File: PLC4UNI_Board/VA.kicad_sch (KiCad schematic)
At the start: 2 parts

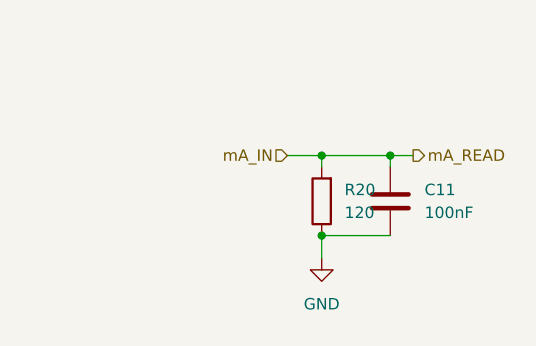
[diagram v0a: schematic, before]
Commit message: v2.1.0
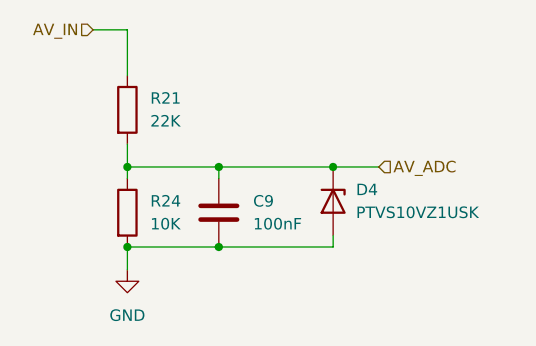
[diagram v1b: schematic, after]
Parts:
- removed C11: 100nF, Capacitor_SMD:C_0805_2012Metric, symbol Device:C
- removed R20: 120, Resistor_SMD:R_0603_1608Metric, symbol Device:R
- added C9: 100nF, Capacitor_SMD:C_0805_2012Metric_Pad1.18x1.45mm_HandSolder, symbol Device:C
- added D4: PTVS10VZ1USK, Diode_SMD:Nexperia_DSN1608-2_1.6x0.8mm, symbol Diode:PTVS10VZ1USK
- added R21: 22K, Resistor_SMD:R_0603_1608Metric, symbol Device:R
- added R24: 10K, Resistor_SMD:R_0603_1608Metric, symbol Device:R
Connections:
- net GND: now also C9.2, D4.2 (A), R24.2
- new net AV_ADC: C9.1, D4.1 (K), R21.2, R24.1
- new net AV_IN: R21.1
